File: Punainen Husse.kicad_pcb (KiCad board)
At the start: 2 copper layers, 99.7 x 77.1 mm, 86 parts, among them Q1 MMBF4393LT1G, Q2 BC807, Q3 MMBF170, Q4 MMBF170, SW1 SW_DPDT_x2, SW2 SW_DPDT_x2, U1 TL074, U2 LF351D, U3 LM13700

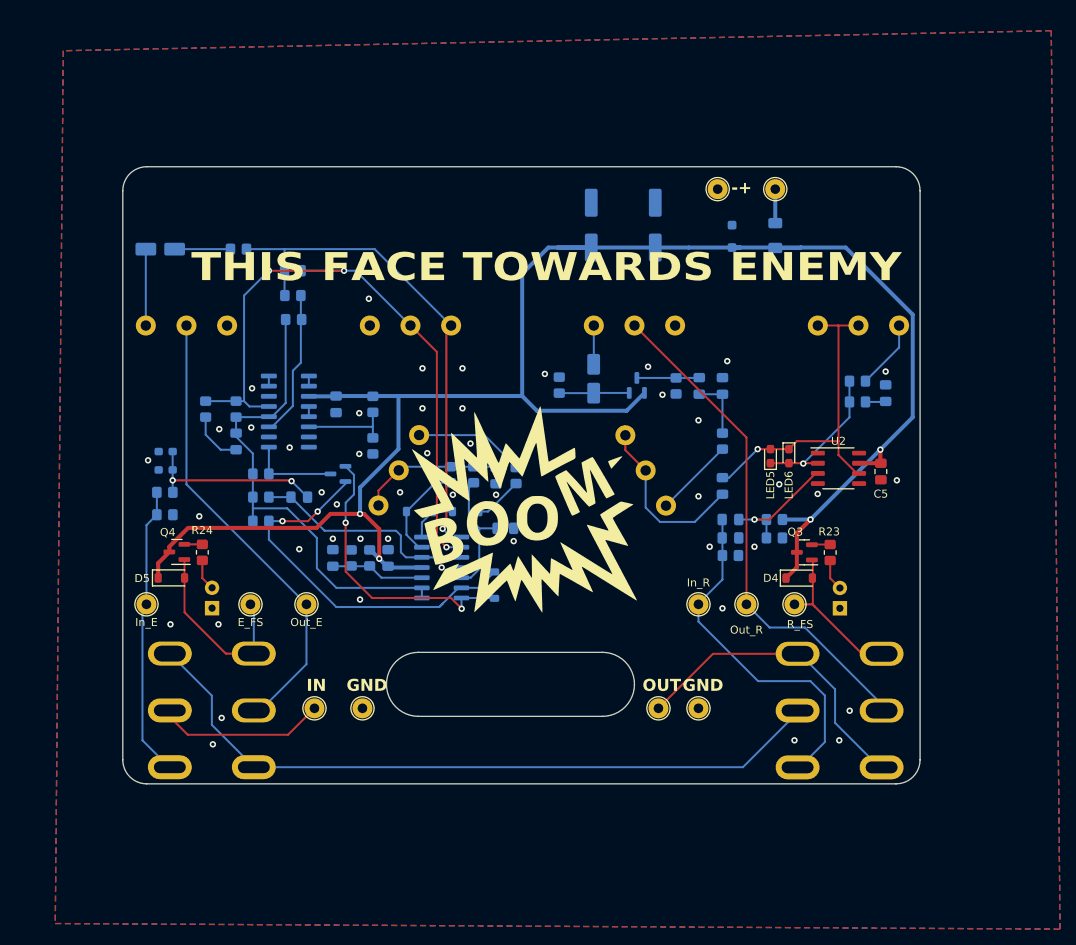
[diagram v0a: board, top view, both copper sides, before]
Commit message: Revision 2
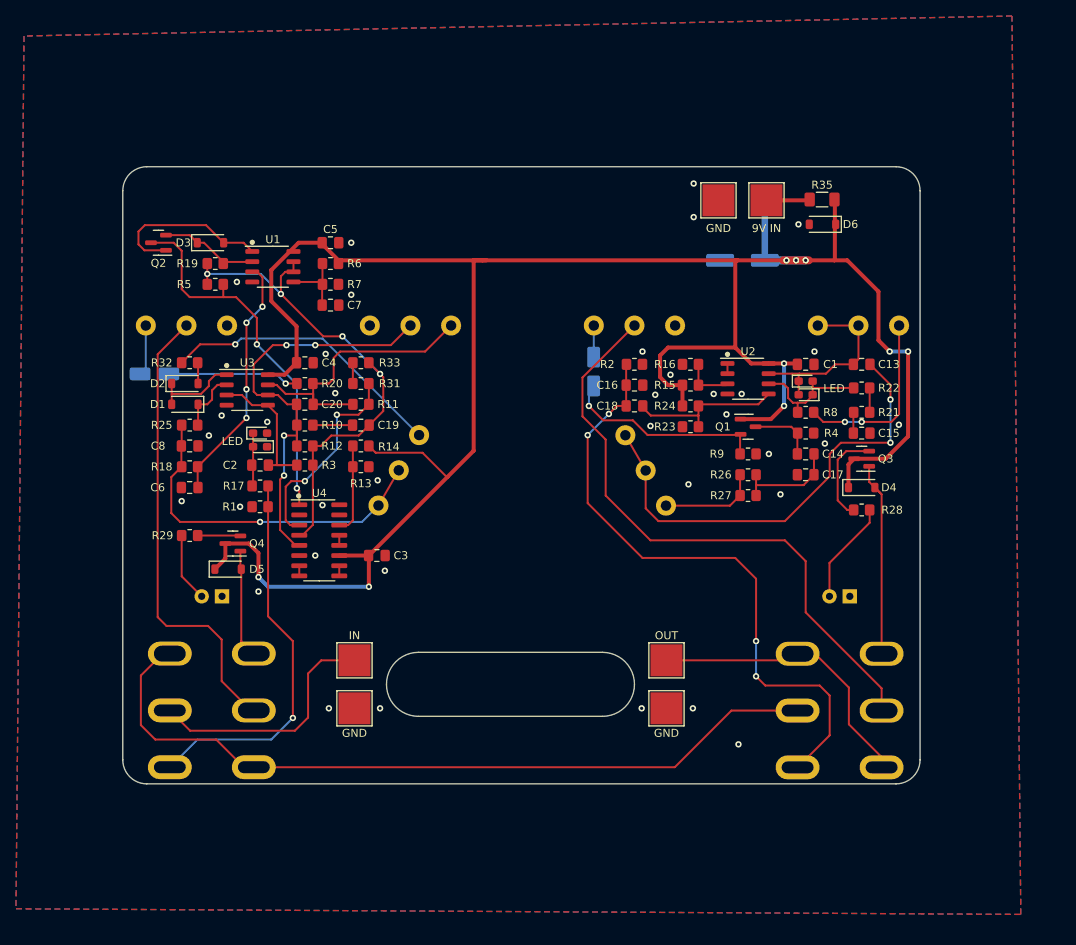
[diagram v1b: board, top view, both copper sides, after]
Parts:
- removed C21: 1uF, Capacitor_SMD:C_0805_2012Metric_Pad1.18x1.45mm_HandSolder
- removed C22, C23: 10nF, Capacitor_SMD:C_0805_2012Metric_Pad1.18x1.45mm_HandSolder
- removed LED5, LED6: LED_Small, LED_SMD:LED_0603_1608Metric_Pad1.05x0.95mm_HandSolder
- removed TP10: In_E, TestPoint:TestPoint_THTPad_D2.5mm_Drill1.2mm
- removed TP5: Out_R, TestPoint:TestPoint_THTPad_D2.5mm_Drill1.2mm
- removed TP6: In_R, TestPoint:TestPoint_THTPad_D2.5mm_Drill1.2mm
- removed TP7: R_FS, TestPoint:TestPoint_THTPad_D2.5mm_Drill1.2mm
- removed TP8: E_FS, TestPoint:TestPoint_THTPad_D2.5mm_Drill1.2mm
- removed TP9: Out_E, TestPoint:TestPoint_THTPad_D2.5mm_Drill1.2mm
- added C13: 100nF, Capacitor_SMD:C_0805_2012Metric_Pad1.18x1.45mm_HandSolder, F.Cu at (199.4, 86.0)
- added C16: 1nF, Capacitor_SMD:C_0805_2012Metric_Pad1.18x1.45mm_HandSolder, F.Cu at (171.0, 88.6)
- added C17: 3.3nF, Capacitor_SMD:C_0805_2012Metric_Pad1.18x1.45mm_HandSolder, F.Cu at (192.4, 99.8)
- added C18: 47nF, Capacitor_SMD:C_0805_2012Metric_Pad1.18x1.45mm_HandSolder, F.Cu at (171.0, 91.2)
- added LED1: LED_Small, LED_SMD:LED_0603_1608Metric_Pad1.05x0.95mm_HandSolder, F.Cu at (192.4, 89.8)
- added LED4: LED_Small, LED_SMD:LED_0603_1608Metric_Pad1.05x0.95mm_HandSolder, F.Cu at (124.2, 94.6)
- added R29: 4.7k, Resistor_SMD:R_0805_2012Metric_Pad1.20x1.40mm_HandSolder, F.Cu at (115.4, 107.4)
- added R31: 100Ω, Resistor_SMD:R_0805_2012Metric_Pad1.20x1.40mm_HandSolder, F.Cu at (136.8, 88.4)
- added R32: 100Ω, Resistor_SMD:R_0805_2012Metric_Pad1.20x1.40mm_HandSolder, F.Cu at (115.4, 85.8)
- added R33: 100Ω, Resistor_SMD:R_0805_2012Metric_Pad1.20x1.40mm_HandSolder, F.Cu at (136.8, 85.8)
- added R35: 39Ω, Resistor_SMD:R_1206_3216Metric_Pad1.30x1.75mm_HandSolder, F.Cu at (194.4, 65.4)
- added U4: LM13700, Package_SO:SOP-16_3.9x9.9mm_P1.27mm, F.Cu at (131.6, 108.0)
- C1: value 1nF -> 10nF; moved to F.Cu
- C10: value 1uF -> 100uF; footprint Capacitor_SMD:C_0805_2012Metric_Pad1.18x1.45mm_HandSolder -> Capacitor_SMD:CP_Elec_6.3x5.4
- C11: value 3.3nF -> 10uF; footprint Capacitor_SMD:C_0805_2012Metric_Pad1.18x1.45mm_HandSolder -> Capacitor_SMD:CP_Elec_4x5.4
- C12: value 100nF -> 10uF; footprint Capacitor_SMD:C_0805_2012Metric_Pad1.18x1.45mm_HandSolder -> Capacitor_SMD:CP_Elec_4x5.4
- C14: value 10uF -> 100nF; footprint Capacitor_SMD:CP_Elec_4x5.4 -> Capacitor_SMD:C_0805_2012Metric_Pad1.18x1.45mm_HandSolder; moved to F.Cu
- C15: value 10uF -> 220nF; footprint Capacitor_SMD:CP_Elec_4x5.4 -> Capacitor_SMD:C_0805_2012Metric_Pad1.18x1.45mm_HandSolder; moved to F.Cu
- C19: value 100uF -> 4.7nF; footprint Capacitor_SMD:CP_Elec_6.3x5.4 -> Capacitor_SMD:C_0805_2012Metric_Pad1.18x1.45mm_HandSolder; moved to F.Cu
- C2: value 47nF -> 10nF; moved to F.Cu
- C20: value 100uF -> 100pF; footprint Capacitor_SMD:CP_Elec_6.3x5.4 -> Capacitor_SMD:C_0805_2012Metric_Pad1.18x1.45mm_HandSolder; moved to F.Cu
- C3, C7, D1, D2, D3, LED2, LED3, Q1, Q2, R1, R10, R12, R2, R21: moved to F.Cu
- C4: value 220nF -> 10nF; moved to F.Cu
- C6: value 4.7nF -> 1uF; moved to F.Cu
- C8: value 100nF -> 1uF; moved to F.Cu
- C9: value 100pF -> 100uF; footprint Capacitor_SMD:C_0805_2012Metric_Pad1.18x1.45mm_HandSolder -> Capacitor_SMD:CP_Elec_6.3x5.4
- D6: footprint Diode_SMD:D_SOD-123F -> Diode_SMD:D_SOD-123; moved to F.Cu
- R11: value 100Ω -> 10k; moved to F.Cu
- R13, R16: value 1k -> 10k; moved to F.Cu
- R14: value 2.2k -> 10k; moved to F.Cu
- R15, R8: value 1M -> 10k; moved to F.Cu
- R17, R19: value 10k -> 1k; moved to F.Cu
- R18: value 1M -> 1k; moved to F.Cu
- R20: value 220Ω -> 1k; moved to F.Cu
- R22: value 39Ω -> 1k; footprint Resistor_SMD:R_1206_3216Metric_Pad1.30x1.75mm_HandSolder -> Resistor_SMD:R_0805_2012Metric_Pad1.20x1.40mm_HandSolder; moved to F.Cu
- R23, R24: value 4.7k -> 470k
- R25: value 10k -> 470k; moved to F.Cu
- R26: value 10k -> 4.7k; moved to F.Cu
- R27, R28: value 1M -> 4.7k; moved to F.Cu
- R3: value 1k -> 1M; moved to F.Cu
- R4, R5: value 470k -> 1M; moved to F.Cu
- R6: value 1.8k -> 1M; moved to F.Cu
- R7: value 10k -> 1M; moved to F.Cu
- R9: value 470k -> 10k; moved to F.Cu
- TP1, TP11, TP12, TP2, TP3, TP4: footprint TestPoint:TestPoint_THTPad_D2.5mm_Drill1.2mm -> TestPoint:TestPoint_Pad_4.0x4.0mm
- U1: value TL074 -> TL072; footprint Package_SO:SO-14_3.9x8.65mm_P1.27mm -> Package_SO:SO-8_3.9x4.9mm_P1.27mm; moved to F.Cu
- U2: value LF351D -> TL072
- U3: value LM13700 -> TL072; footprint Package_SO:SOP-16_3.9x9.9mm_P1.27mm -> Package_SO:SO-8_3.9x4.9mm_P1.27mm; moved to F.Cu
- moved C15 90.6 mm to (199.4, 94.6), turned to 0 degrees
- moved LED2 80.8 mm to (192.4, 88.1), turned to 0 degrees
- moved R21 80.5 mm to (199.4, 92.0)
- moved R5 76.8 mm to (118.6, 76.0)
- moved C5 74.5 mm to (133.0, 70.8), turned to 0 degrees
- moved C4 72.7 mm to (129.8, 85.8), turned to 0 degrees
- moved R8 68.9 mm to (192.4, 92.0), turned to 180 degrees
- moved C12 68.1 mm to (111.0, 87.2), turned to 180 degrees
- moved R6 68.1 mm to (133.0, 73.4), turned to 180 degrees
- moved R7 67.0 mm to (133.0, 76.0), turned to 0 degrees
- moved C8 66.8 mm to (115.4, 96.2), turned to 0 degrees
- moved R28 64.1 mm to (199.4, 104.2), turned to 0 degrees
- moved R24 63.7 mm to (178.0, 91.2), turned to 0 degrees
- moved C2 59.2 mm to (124.2, 98.6), turned to 180 degrees
- moved R16 57.2 mm to (178.0, 86.0), turned to 180 degrees
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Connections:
- C1 pad 1: IN_red_pcb -> +9V
- C10 pad 1: Net-(U1D-+) -> +9V
- C11 pad 1: Net-(C11-Pad1) -> Net-(Q1-S)
- C11 pad 2: GND -> Net-(C11-Pad2)
- C12 pad 1: Net-(Q1-G) -> Net-(C12-Pad1)
- C12 pad 2: Net-(C11-Pad1) -> Net-(C12-Pad2)
- C14 pad 1: Net-(Q1-S) -> Net-(Q1-G)
- C15 pad 2: Net-(C15-Pad2) -> GND
- C19 pad 1: +9V -> Net-(C19-Pad1)
- C19 pad 2: GND -> +5V
- C2 pad 1: IN_red_pcb -> Net-(U3A-+)
- C2 pad 2: Net-(U2-+) -> Net-(LED3-A)
- C20 pad 1: +9V -> Net-(C20-Pad1)
- C20 pad 2: GND -> Net-(U3B--)
- C3 pad 1: Net-(U1B-+) -> +9V
- C3 pad 2: Net-(LED2-K) -> GND
- C4 pad 1: Net-(C4-Pad1) -> +9V
- C6 pad 1: Net-(C6-Pad1) -> Net-(U1A-+)
- C6 pad 2: +5V -> GND
- C7 pad 1: Net-(C7-Pad1) -> GND
- C7 pad 2: GND -> Net-(U1B-+)
- C8 pad 2: Net-(LED5-A) -> GND
- C9 pad 1: Net-(C9-Pad1) -> +9V
- C9 pad 2: Net-(U1C--) -> GND
- LED2 pad 1: Net-(LED2-K) -> Net-(LED1-A)
- LED2 pad 2: GND -> Net-(LED1-K)
- LED3 pad 2: Net-(LED2-K) -> Net-(LED3-A)
- R10 pad 1: Net-(C6-Pad1) -> Net-(C19-Pad1)
- R10 pad 2: Net-(U1C--) -> Net-(U3B--)
- R11 pad 1: Net-(D2-A) -> Net-(U4C-+)
- R11 pad 2: Net-(R11-Pad2) -> Net-(C20-Pad1)
- R12 pad 2: Net-(U1C--) -> Net-(U3B--)
- R13 pad 1: Net-(C7-Pad1) -> Net-(U4A-+)
- R13 pad 2: Net-(U1D-+) -> GND
- R14 pad 1: Net-(R14-Pad1) -> +9V
- R14 pad 2: Net-(C11-Pad1) -> Net-(U4A-+)
- R15 pad 1: Net-(Q1-G) -> +9V
- R15 pad 2: GND -> Net-(U2A-+)
- R16 pad 1: +5V -> Net-(U2A-+)
- R16 pad 2: Net-(D3-K) -> GND
- R17 pad 1: Net-(Q1-S) -> IN_engi_pcb
- R17 pad 2: GND -> Net-(LED3-A)
- R18 pad 1: +5V -> Net-(C8-Pad1)
- R18 pad 2: Net-(Q2-C) -> Net-(U1A-+)
- R19 pad 1: Net-(U3C-+) -> +5V
- R19 pad 2: Net-(C9-Pad1) -> Net-(D3-K)
- R20 pad 1: +5V -> Net-(C20-Pad1)
- R20 pad 2: Net-(U3C-+) -> Net-(C12-Pad1)
- R21 pad 1: Net-(C9-Pad1) -> Net-(R21-Pad1)
- R22 pad 1: Net-(R22-Pad1) -> Net-(R21-Pad1)
- R22 pad 2: +9V -> Net-(LED1-K)
- R23 pad 1: Net-(Q3-S) -> Net-(U2B-+)
- R23 pad 2: Net-(LED7-A) -> GND
- R24 pad 1: Net-(Q4-S) -> +9V
- R24 pad 2: Net-(LED8-A) -> Net-(U2B-+)
- R25 pad 1: +9V -> Net-(C8-Pad1)
- R25 pad 2: Net-(U3A-+) -> Net-(D1-K)
- R26 pad 1: Net-(U3A-+) -> Net-(C14-Pad2)
- R26 pad 2: GND -> Net-(R26-Pad2)
- R27 pad 1: +9V -> Net-(C14-Pad2)
- R27 pad 2: Net-(U1A-+) -> Net-(R26-Pad2)
- R28 pad 1: Net-(U1A-+) -> Net-(Q3-S)
- R28 pad 2: GND -> Net-(LED7-A)
- R3 pad 1: IN_engi_pcb -> +5V
- R3 pad 2: Net-(LED2-K) -> Net-(U3A-+)
- R4 pad 1: +9V -> Net-(Q1-G)
- R4 pad 2: Net-(U2-+) -> GND
- R5 pad 1: Net-(U2-+) -> +5V
- R5 pad 2: GND -> Net-(Q2-C)
- R6 pad 1: Net-(LED5-K) -> +9V
- R6 pad 2: Net-(C4-Pad1) -> Net-(U1B-+)
- R7 pad 1: Net-(R7-Pad1) -> Net-(U1B-+)
- R7 pad 2: Net-(LED5-K) -> GND
- R8 pad 1: +5V -> Net-(R8-Pad1)
- R8 pad 2: Net-(U1B-+) -> Net-(LED1-K)
- R9 pad 1: Net-(C7-Pad1) -> Net-(Q1-S)
- R9 pad 2: Net-(D1-K) -> GND
- Rv1 pad 1: Net-(R7-Pad1) -> Net-(R8-Pad1)
- Rv1 pad 2: Net-(LED5-A) -> Net-(LED1-A)
- Rv1 pad 3: Net-(LED5-A) -> Net-(LED1-A)
- Rv2 pad 1: Net-(R14-Pad1) -> Net-(R26-Pad2)
- Rv2 pad 2: Net-(C8-Pad1) -> Net-(C13-Pad1)
- Rv2 pad 3: Net-(C8-Pad1) -> Net-(C13-Pad1)
- Rv3 pad 3: Net-(C14-Pad2) -> Net-(C11-Pad2)
- Rv4 pad 1: Net-(R11-Pad2) -> Net-(R32-Pad2)
- Rv4 pad 2: Net-(C7-Pad1) -> Net-(C8-Pad1)
- Rv4 pad 3: Net-(C7-Pad1) -> Net-(C8-Pad1)
- Rv5 pad 1: Net-(C9-Pad1) -> Net-(C20-Pad1)
- Rv5 pad 2: Net-(U1C--) -> Net-(U3B--)
- Rv6 pad 3: Net-(C15-Pad2) -> Net-(C12-Pad2)
- TP12 pad 1: Net-(R22-Pad1) -> 9V in
- U1 pad 1: +5V -> Net-(D3-A)
- U1 pad 2: +5V -> Net-(D3-K)
- U1 pad 4: +9V -> GND
- U1 pad 6: Net-(D1-K) -> +5V
- U1 pad 7: Net-(D1-A) -> +5V
- U1 pad 8: Net-(C9-Pad1) -> +9V
- U2 pad 1: unconnected-(U2-NULL-Pad1) -> Net-(U2A--)
- U2 pad 2: Net-(LED5-K) -> Net-(U2A--)
- U2 pad 3: Net-(U2-+) -> Net-(U2A-+)
- U2 pad 5: unconnected-(U2-NULL-Pad5) -> Net-(U2B-+)
- U2 pad 6: Net-(LED5-A) -> Net-(LED1-K)
- U2 pad 7: +9V -> Net-(LED1-A)
- U2 pad 8: unconnected-(U2-NC-Pad8) -> +9V
- U3 pad 1: Net-(Q2-C) -> Net-(D1-A)
- U3 pad 2: unconnected-(U3C-DIODE_BIAS-Pad2) -> Net-(D1-K)
- U3 pad 3: Net-(U3C-+) -> Net-(U3A-+)
- U3 pad 4: +5V -> GND
- U3 pad 5: Net-(U1C--) -> Net-(U3A-+)
- U3 pad 6: GND -> Net-(U3B--)
- U3 pad 7: Net-(U3-Pad7) -> Net-(C20-Pad1)
- U3 pad 8: Net-(U3-Pad7) -> +9V
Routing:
- net Net-(U1C--): track 83.1 -> 0.00 mm, vias 3 -> 0
- net Net-(C9-Pad1): track 64.0 -> 0.00 mm, vias 1 -> 0
- net +9V: track 229.4 -> 289.3 mm, vias 4 -> 9
- net Net-(C13-Pad1): track 0.00 -> 57.6 mm, vias 0 -> 2
- net Net-(U3B--): track 0.00 -> 53.1 mm, vias 0 -> 4
- net Net-(LED5-A): track 41.2 -> 0.00 mm, vias 1 -> 0
- net Net-(C20-Pad1): track 0.00 -> 36.8 mm
- net Net-(Q2-C): track 11.1 -> 47.1 mm, vias 0 -> 2
- net Net-(R32-Pad2): track 0.00 -> 35.9 mm, vias 0 -> 1
- net Net-(D3-K): track 48.1 -> 12.5 mm, vias 2 -> 0
- net IN_red_pcb: track 43.9 -> 77.8 mm, vias 0 -> 4
- net Net-(U4C-+): track 0.00 -> 25.9 mm, vias 0 -> 2
- net Net-(LED1-A): track 0.00 -> 23.9 mm
- net Net-(LED2-K): track 22.8 -> 0.00 mm, vias 2 -> 0
- net Net-(R8-Pad1): track 0.00 -> 22.7 mm, vias 0 -> 2
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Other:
- board text added: "LED"
- board text added: "https://github.com/Secret624/punainenHusse"
- board text added: "rev. 2"
- board text removed: "-+"
- board text removed: "GND"
- board text removed: "IN"
- board text removed: "OUT"
- board text removed: "Rev. 2"
- board text removed: "THIS FACE TOWARDS ENEMY"
